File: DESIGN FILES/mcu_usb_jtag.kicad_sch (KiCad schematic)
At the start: 24 parts

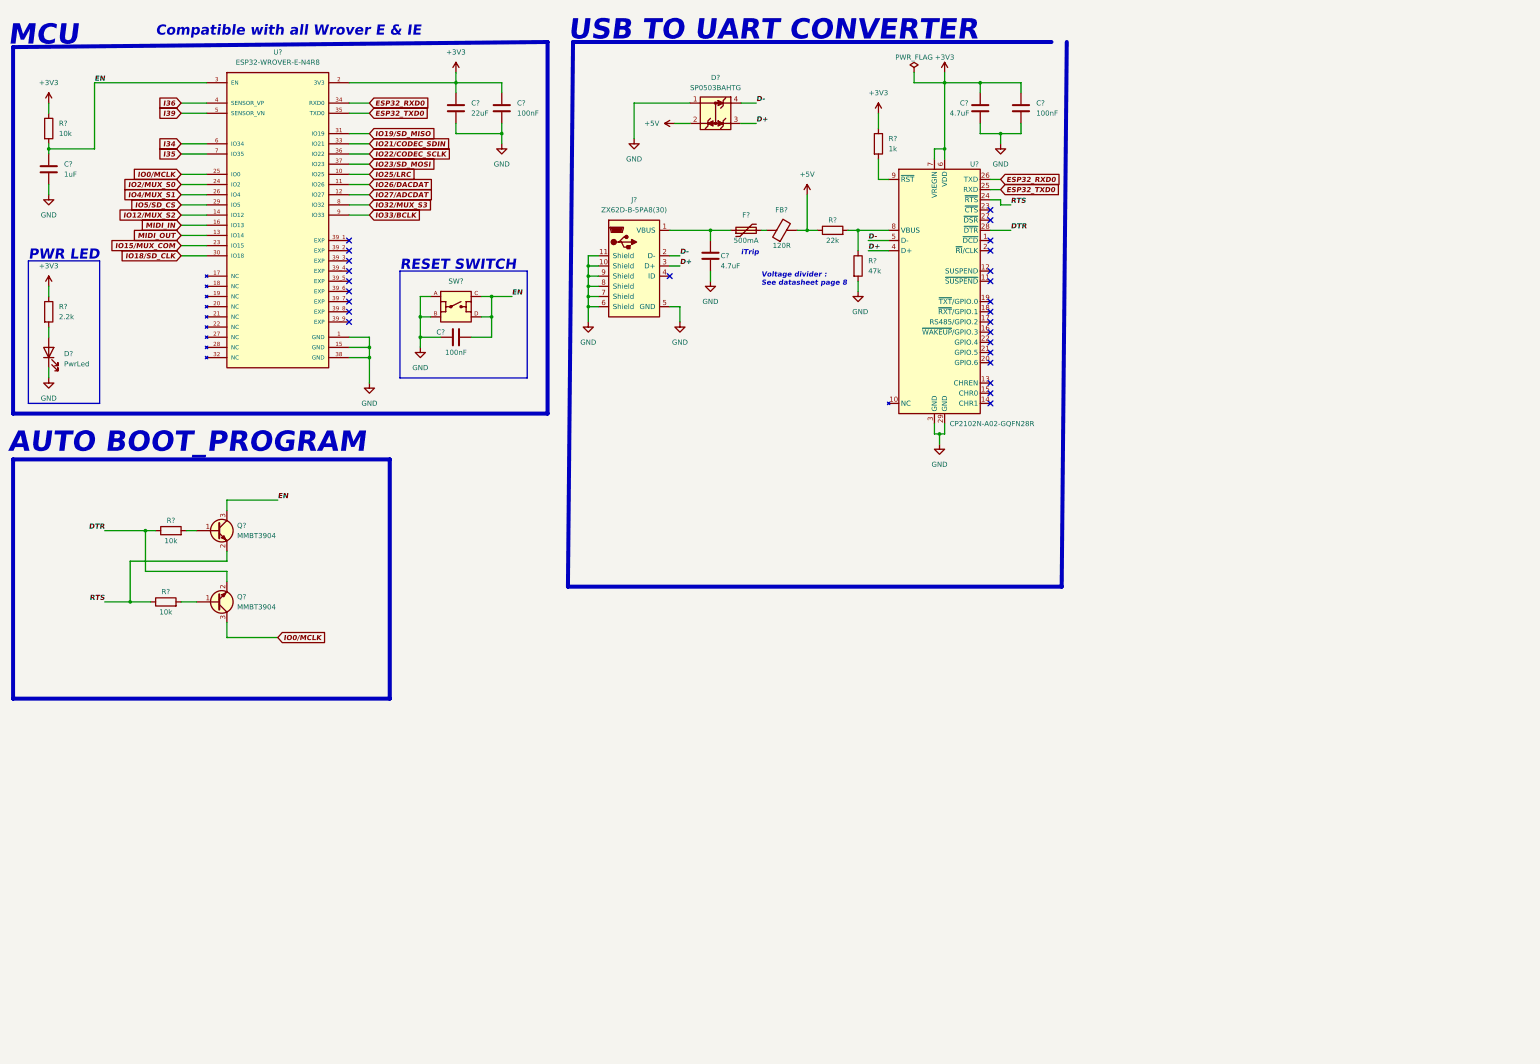
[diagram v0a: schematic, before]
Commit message: updates
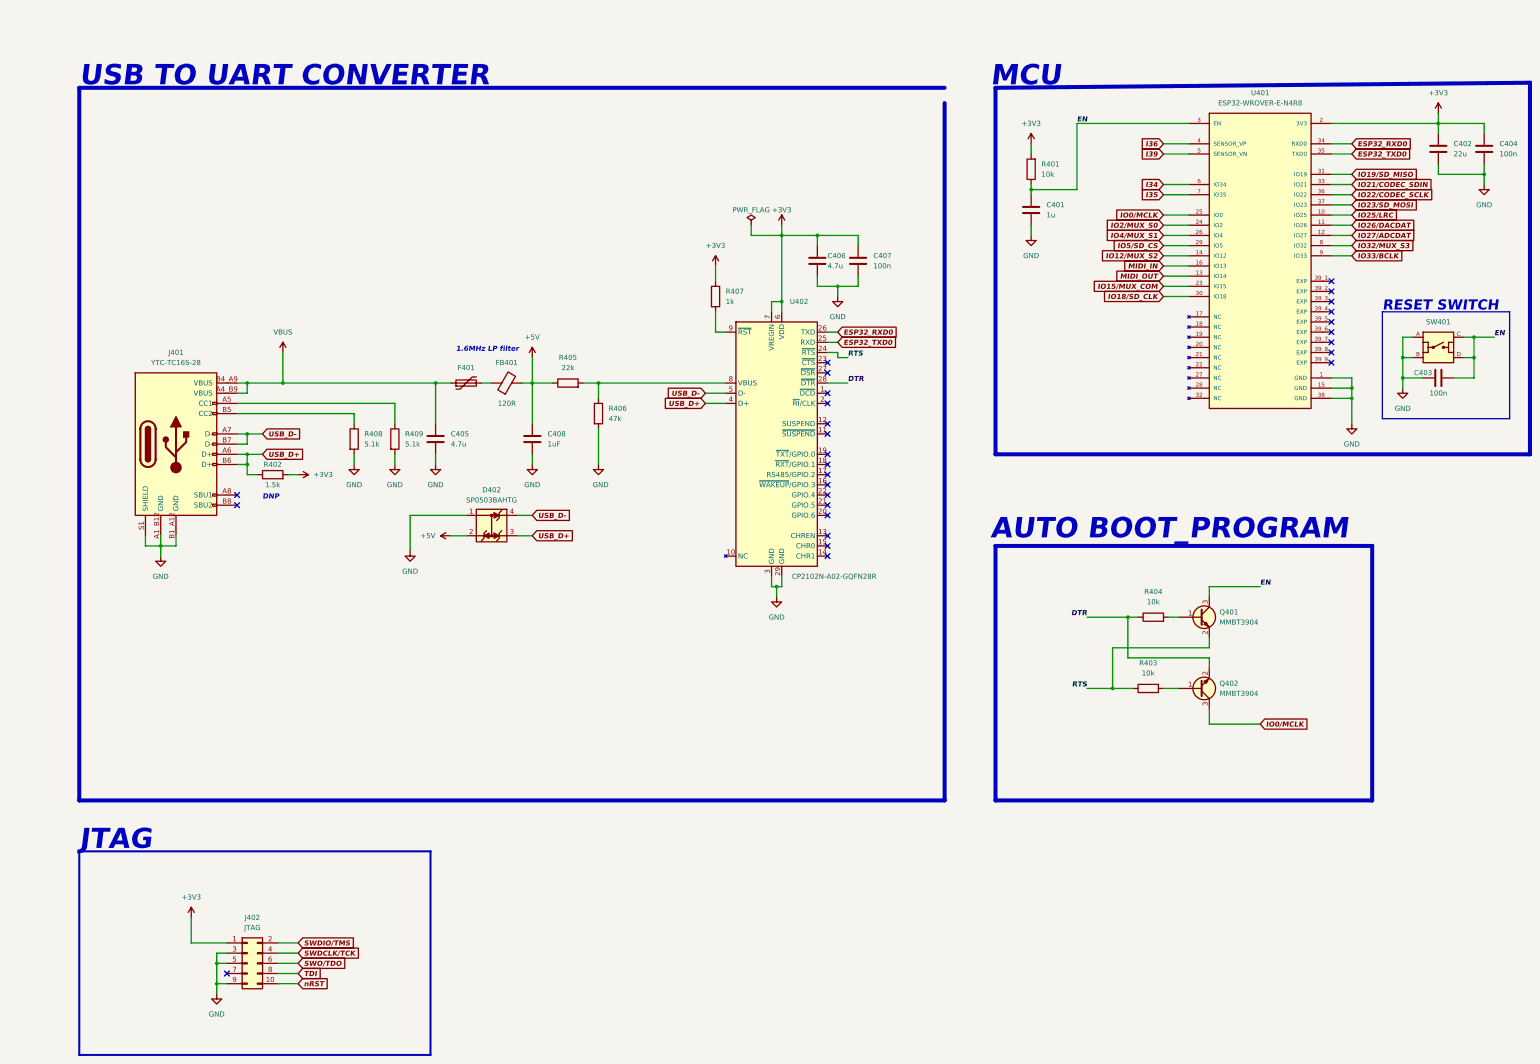
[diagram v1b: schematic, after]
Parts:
- removed C? (x2): 4.7uF, soundsom:CL10A475KO8NNNC_0603, symbol soundsom:CL10A475KO8NNNC
- removed C?: 1uF, soundsom:CL10A105KB8NNNC_0603, symbol soundsom:CL10A105KB8NNNC
- removed C? (x3): 100nF, soundsom:CC0603KRX7R9BB104_0603, symbol soundsom:CC0603KRX7R9BB104
- removed C?: 22uF, soundsom:CL10A226MQ8NRNC_0603, symbol soundsom:CL10A226MQ8NRNC
- removed D?: PwrLed, soundsom:19-217_GHC-YR1S2_3T_0603, symbol soundsom:19-217_GHC-YR1S2_3T
- removed D?: SP0503BAHTG, soundsom:SP0503BAHTG_SOT-143, symbol soundsom:SP0503BAHTG
- removed F?: 500mA, soundsom:SMD0805P020TF_0805, symbol soundsom:SMD0805P020TF
- removed FB?: 120R, soundsom:BLM18AG121SN1D_0603, symbol soundsom:BLM18AG121SN1D
- removed J?: ZX62D-B-5PA8(30), soundsom:ZX62D-B-5PA8(30)_smd, symbol soundsom:ZX62D-B-5PA8(30)
- removed Q? (x2): MMBT3904, soundsom:MMBT3904_SOT-23, symbol soundsom:MMBT3904
- removed R? (x3): 10k, soundsom:0603WAF1002T5E_0603, symbol soundsom:0603WAF1002T5E
- removed R?: 2.2k, soundsom:0603WAF2201T5E_0603, symbol soundsom:0603WAF2201T5E
- removed R?: 1k, soundsom:0603WAF1001T5E_0603, symbol soundsom:0603WAF1001T5E
- removed R?: 22k, soundsom:0603WAF2202T5E_0603, symbol soundsom:0603WAF2202T5E
- removed R?: 47k, soundsom:0603WAF4702T5E_0603, symbol soundsom:0603WAF4702T5E
- removed SW?: TS-1187A-B-A-B, soundsom:TS-1187A-B-A-B_smd, symbol soundsom:TS-1187A-B-A-B
- removed U?: ESP32-WROVER-E-N4R8, soundsom:XCVR_ESP32-WROVER-E-N4R8, symbol soundsom:ESP32-WROVER-E-N4R8
- removed U?: CP2102N-A02-GQFN28R, soundsom:CP2102N-A02-GQFN28R_QFN-28, symbol soundsom:CP2102N-A02-GQFN28R
- added C401: 1u, MY CAPACITOR LIBRARY:CL10A105KB8NNNC_0603, symbol MY CAPACITOR LIBRARY:CL10A105KB8NNNC
- added C402: 22u, MY CAPACITOR LIBRARY:0603_CL10A226MQ8NRNC, symbol MY CAPACITOR LIBRARY:CL10A226MQ8NRNC
- added C403, C404, C407: 100n, MY CAPACITOR LIBRARY:CC0603KRX7R9BB104_0603, symbol MY CAPACITOR LIBRARY:CC0603KRX7R9BB104
- added C405, C406: 4.7u, MY CAPACITOR LIBRARY:CL10A475KO8NNNC_0603, symbol MY CAPACITOR LIBRARY:CL10A475KO8NNNC
- added C408: 1uF, MY CAPACITOR LIBRARY:CL10A105KB8NNNC_0603, symbol MY CAPACITOR LIBRARY:CL10A105KB8NNNC
- added D402: SP0503BAHTG, MY DIODE LIBRARY:SP0503BAHTG_SOT-143, symbol MY DIODE LIBRARY:SP0503BAHTG
- added F401: SMD0805P020TF, MY FUSE LIBRARY:0805_SMD0805P020TF, symbol MY FUSE LIBRARY:SMD0805P020TF
- added FB401: 120R, MY FERRITE BEAD LIBRARY:0603_BLM18AG121SN1D, symbol MY FERRITE BEAD LIBRARY:BLM18AG121SN1D
- added J401: YTC-TC16S-28, MY CONNECTOR LIBRARY:YTC-TC16S-28, symbol MY CONNECTOR LIBRARY:YTC-TC16S-28
- added J402: JTAG, MY CONNECTOR LIBRARY:PZ127VS-12-10-H10-A38, symbol MY CONNECTOR LIBRARY:PZ127VS-12-10-H10-A38
- added Q401, Q402: MMBT3904, MY TRANSISTOR LIBRARY:MMBT3904_SOT-23, symbol MY TRANSISTOR LIBRARY:MMBT3904
- added R401, R403, R404: 10k, MY RESISTOR LIBRARY:0603WAF1002T5E, symbol MY RESISTOR LIBRARY:0603WAF1002T5E
- added R402: 1.5k, MY RESISTOR LIBRARY:CQ03WAJ0152T5E, symbol MY RESISTOR LIBRARY:CQ03WAJ0152T5E
- added R405: 22k, MY RESISTOR LIBRARY:0603WAF2202T5E, symbol MY RESISTOR LIBRARY:0603WAF2202T5E
- added R406: 47k, MY RESISTOR LIBRARY:0603WAF4702T5E, symbol MY RESISTOR LIBRARY:0603WAF4702T5E
- added R407: 1k, MY RESISTOR LIBRARY:0603WAF1001T5E, symbol MY RESISTOR LIBRARY:0603WAF1001T5E
- added R408, R409: 5.1k, MY RESISTOR LIBRARY:0603WAF5101T5E, symbol MY RESISTOR LIBRARY:0603WAF5101T5E
- added SW401: TS-1187A-B-A-B, MY SWITCH LIBRARY:TS-1187A-B-A-B_smd, symbol MY SWITCH LIBRARY:TS-1187A-B-A-B
- added U401: ESP32-WROVER-E-N4R8, MY MICROCONTROLLER LIBRARY:XCVR_ESP32-WROVER-E-N4R8, symbol MY MICROCONTROLLER LIBRARY:ESP32-WROVER-E-N4R8
- added U402: CP2102N-A02-GQFN28R, MY IC LIBRARY:CP2102N-A02-GQFN28R_QFN-28, symbol MY IC LIBRARY:CP2102N-A02-GQFN28R
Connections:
- net +3V3: now also C402.1, C404.1, C406.1, C407.1, J402.1 (Pin_1), R401.2, R402.2, R407.1, U401.2 (3V3), U402.6 (VDD), U402.7 (VREGIN)
- net +5V: now also C408.1, D402.2, FB401.2, R405.1
- net DTR: now also Q402.2 (E), R404.1, U402.28 (~{DTR})
- net EN: now also C401.1, C403.2, Q401.3 (C), R401.1, SW401.C, SW401.D, U401.3 (EN)
- net ESP32_RXD0: now also U401.34 (RXD0), U402.26 (TXD)
- net ESP32_TXD0: now also U401.35 (TXD0), U402.25 (RXD)
- net GND: now also C401.2, C402.2, C403.1, C404.2, C405.2, C406.2, C407.2, C408.2, D402.1, J401.A1_B12 (GND), J401.B1_A12 (GND), J401.S1 (SHIELD), J402.3 (Pin_3), J402.5 (Pin_5), J402.9 (Pin_9), R406.2, R408.2, R409.2, SW401.A, SW401.B, U401.1 (GND), U401.15 (GND), U401.38 (GND), U402.29 (GND), U402.3 (GND)
- net I34: now also U401.6 (IO34)
- net I35: now also U401.7 (IO35)
- net I36: now also U401.4 (SENSOR_VP)
- net I39: now also U401.5 (SENSOR_VN)
- net IO0/MCLK: now also Q402.3 (C), U401.25 (IO0)
- net IO12/MUX_S2: now also U401.14 (IO12)
- net IO15/MUX_COM: now also U401.23 (IO15)
- net IO18/SD_CLK: now also U401.30 (IO18)
- net IO19/SD_MISO: now also U401.31 (IO19)
- net IO21/CODEC_SDIN: now also U401.33 (IO21)
- net IO22/CODEC_SCLK: now also U401.36 (IO22)
- net IO23/SD_MOSI: now also U401.37 (IO23)
- net IO25/LRC: now also U401.10 (IO25)
- net IO26/DACDAT: now also U401.11 (IO26)
- net IO27/ADCDAT: now also U401.12 (IO27)
- net IO2/MUX_S0: now also U401.24 (IO2)
- net IO32/MUX_S3: now also U401.8 (IO32)
- net IO33/BCLK: now also U401.9 (IO33)
- net IO4/MUX_S1: now also U401.26 (IO4)
- net IO5/SD_CS: now also U401.29 (IO5)
- net MIDI_IN: now also U401.16 (IO13)
- net MIDI_OUT: now also U401.13 (IO14)
- net RTS: now also Q401.2 (E), R403.1, U402.24 (~{RTS})
- new net: Q402.1 (B), R403.2
- new net: J401.B5 (CC2), R408.1
- new net: Q401.1 (B), R404.2
- new net: F401.2, FB401.1
- new net: R405.2, R406.1, U402.8 (VBUS)
- new net: R407.2, U402.9 (~{RST})
- new net: J401.A5 (CC1), R409.1
- new net SWDCLK/TCK: J402.4 (Pin_4)
- new net SWDIO/TMS: J402.2 (Pin_2)
- new net SWO/TDO: J402.6 (Pin_6)
- new net TDI: J402.8 (Pin_8)
- new net USB_D+: D402.3, J401.A6 (D+), J401.B6 (D+), R402.1, U402.4 (D+)
- new net USB_D-: D402.4, J401.A7 (D-), J401.B7 (D-), U402.5 (D-)
- new net VBUS: C405.1, F401.1, J401.A4_B9 (VBUS), J401.B4_A9 (VBUS)
- new net nRST: J402.10 (Pin_10)
- no-connect marks 26 -> 28
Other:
- note added: "1.6MHz LP filter"
- note added: "DNP"
- note added: "JTAG"
- note removed: "Compatible with all Wrover E & IE"
- note removed: "PWR LED"
- note removed: "Voltage divider : See datasheet page 8"
- note removed: "iTrip"
